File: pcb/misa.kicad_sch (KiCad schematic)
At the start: 41 parts, among them J1 PLD JTAG, J2 UART, J3 CF CARD, J4 44 PIN IDE, SW1 Reset, U1 MC68000P, U11 SST39SF040, U12 SST39SF040, U2 NE555P, U3 ATF1508ASx-xxJx84, U4 74HC74, U5 74LS05, U7 AS6C4008-55PCN, U8 AS6C4008-55PCN, U9 TL16C550DPTR, Y1 8MHz, Y2 1.8432MHz

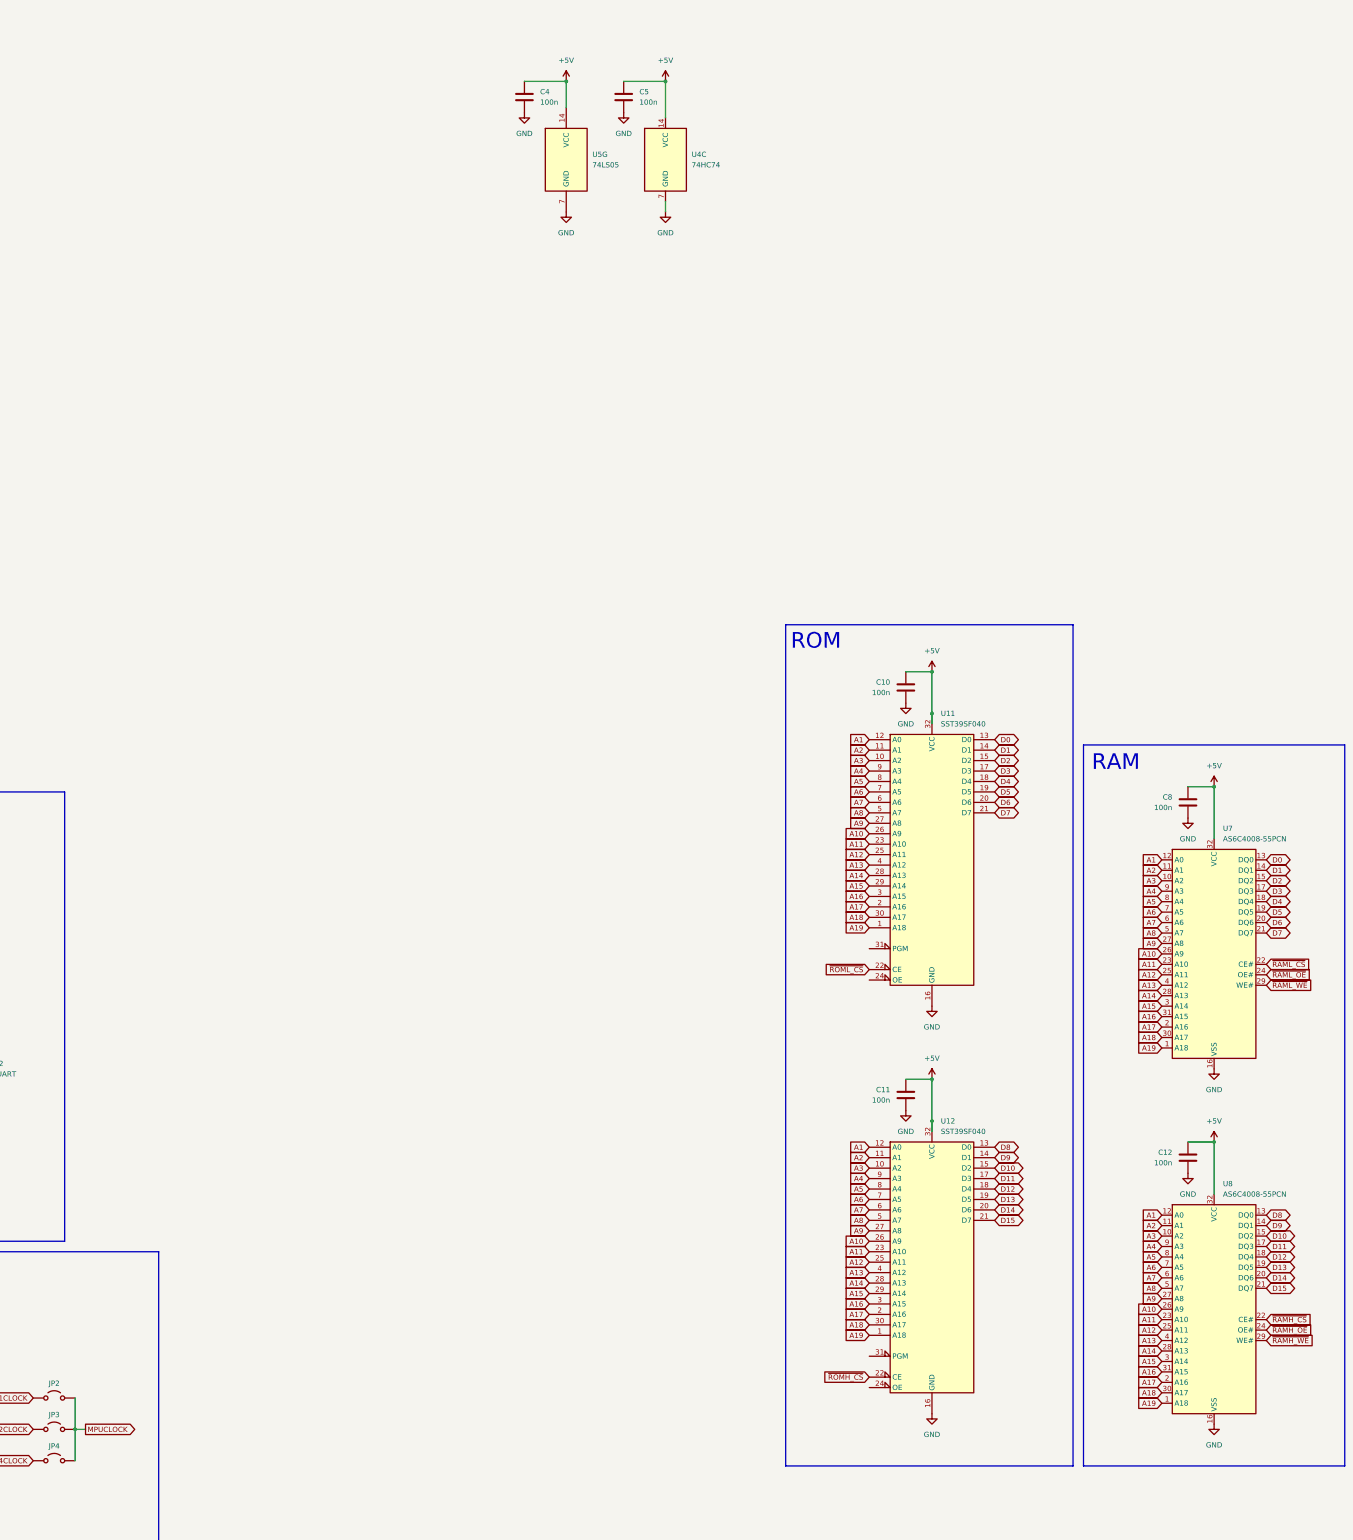
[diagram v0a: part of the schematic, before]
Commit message: stuff
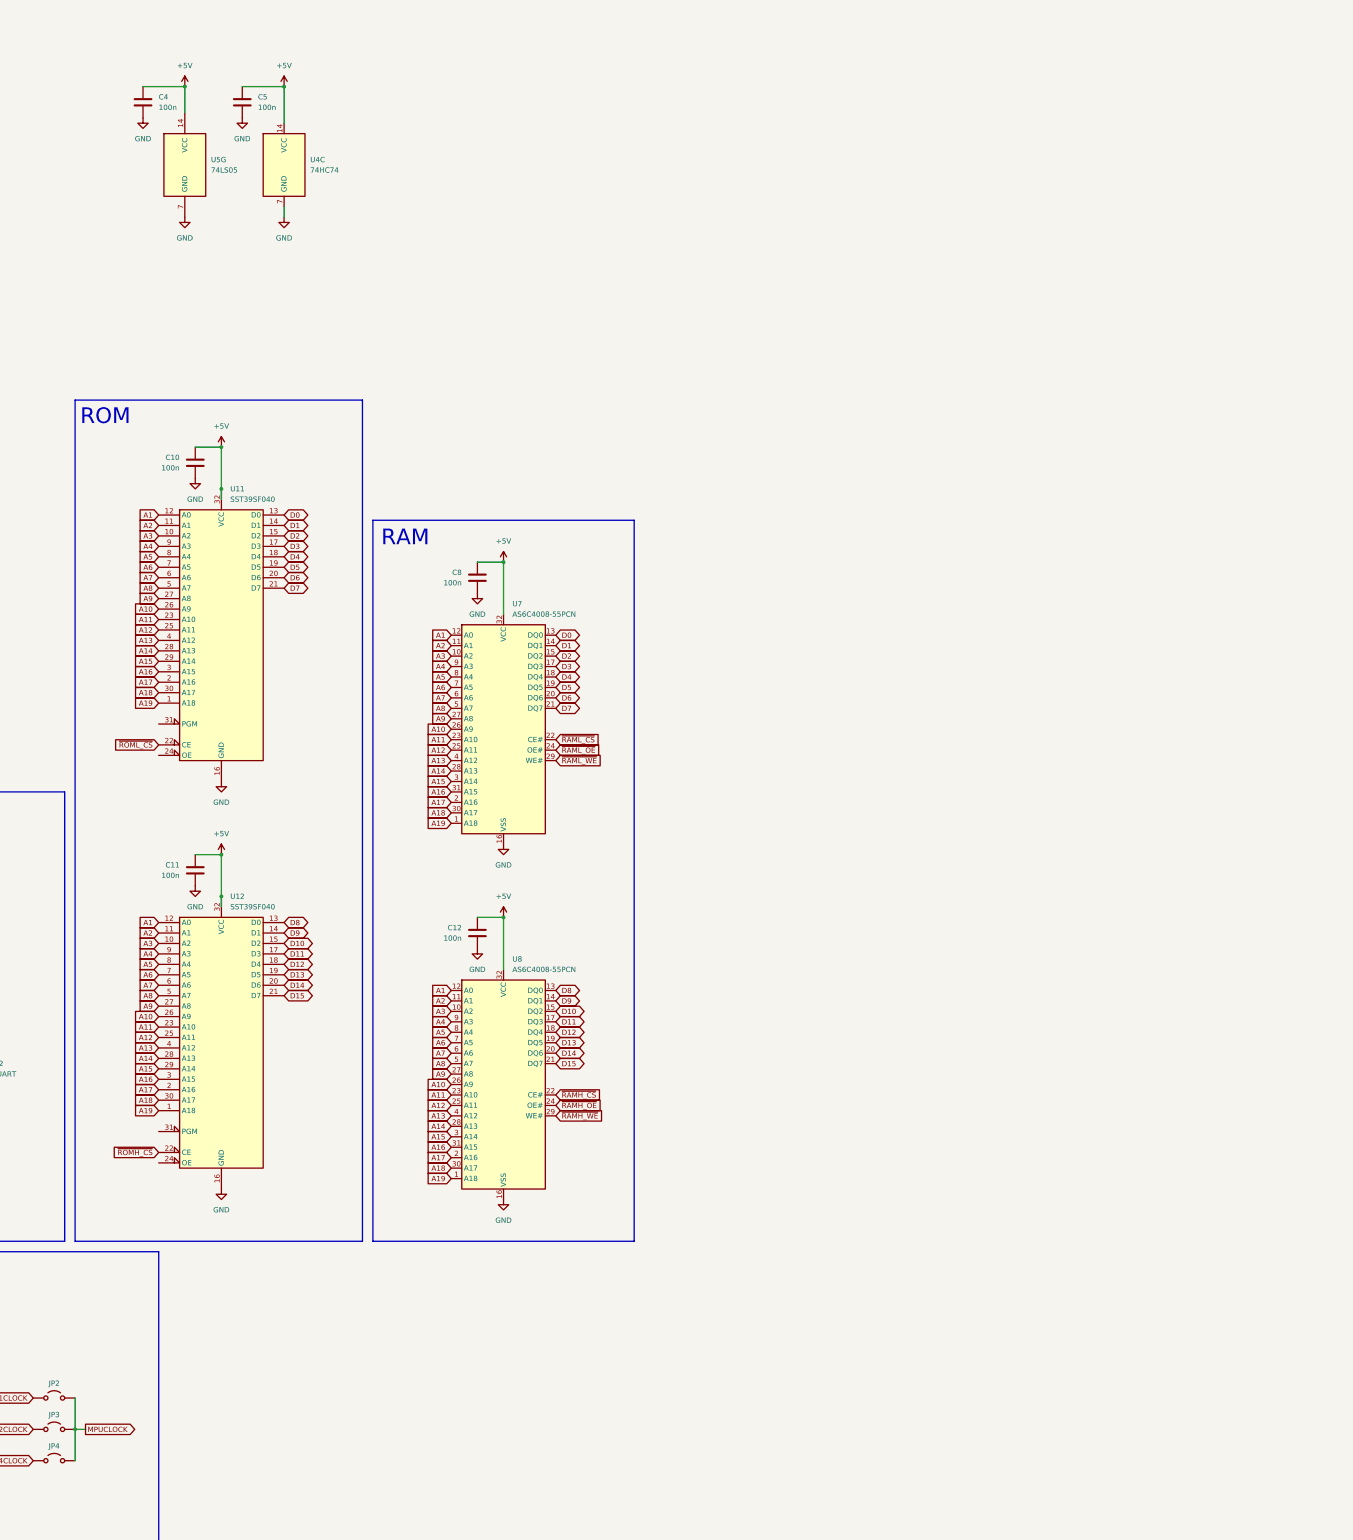
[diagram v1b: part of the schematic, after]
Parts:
- added unit 7 of U5
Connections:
- net +5V: now also U5.14 (VCC); no longer U5.14 (VCC)
- net GND: now also U5.7 (GND); no longer U5.7 (GND)
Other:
- moved on the sheet: C10, C11, C12, C4, C5, C8, U11, U12, U4C, U7, U8
